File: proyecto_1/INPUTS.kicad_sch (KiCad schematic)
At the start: 28 parts, among them U10 FODM2705, U7 FODM2705, U8 FODM2705, U9 FODM2705

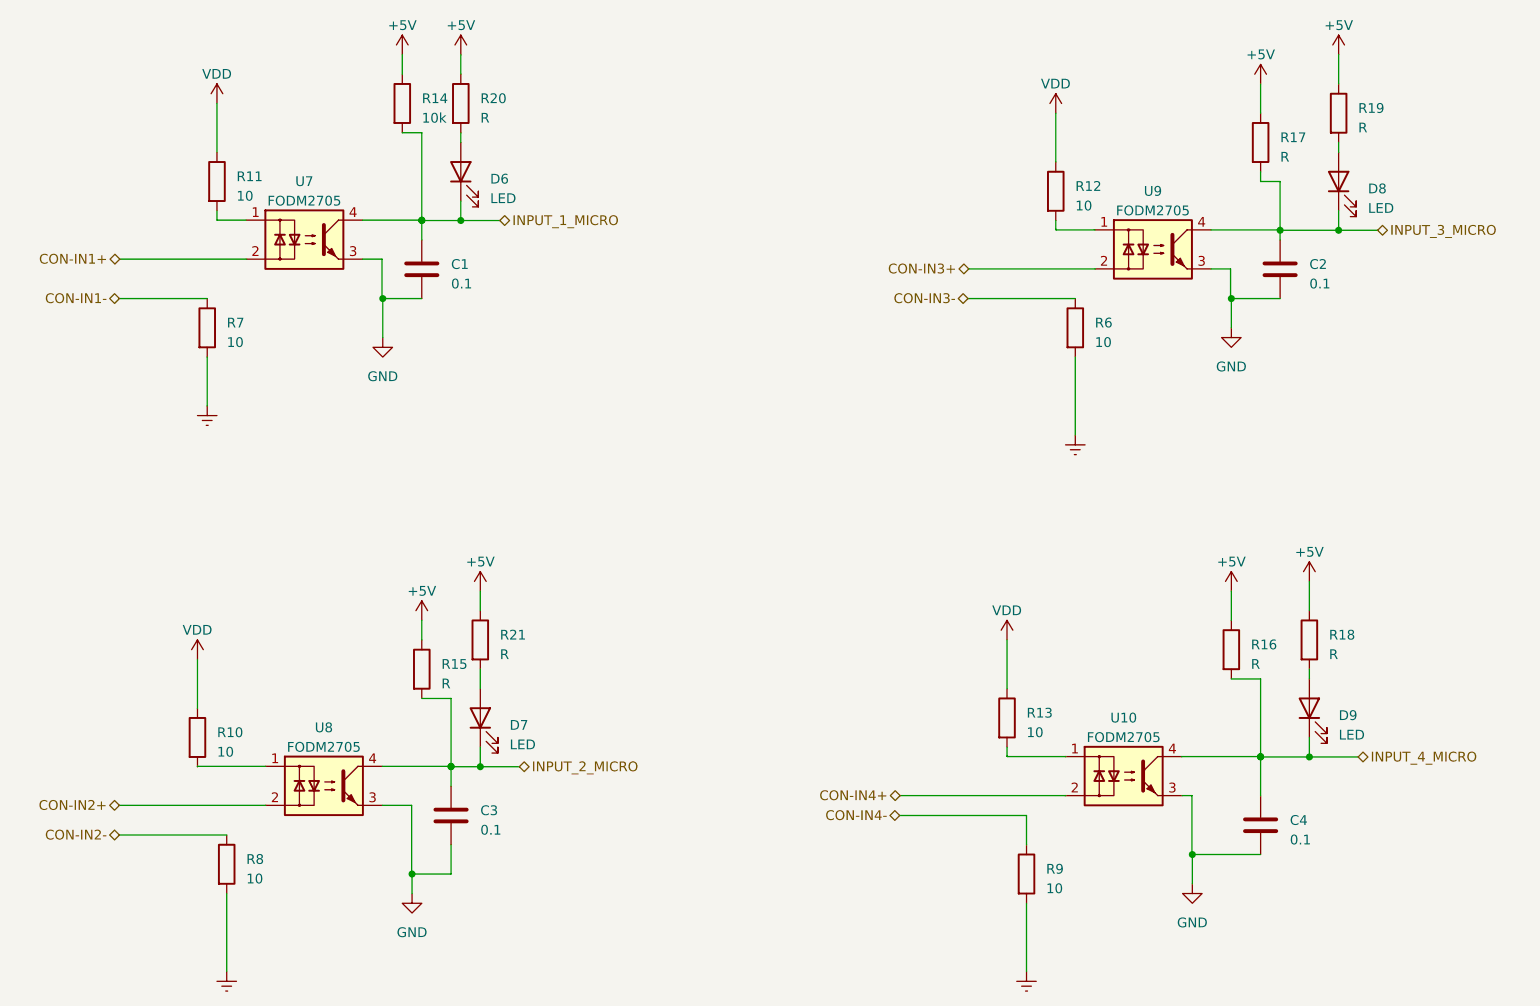
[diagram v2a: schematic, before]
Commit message: avance del proyecto
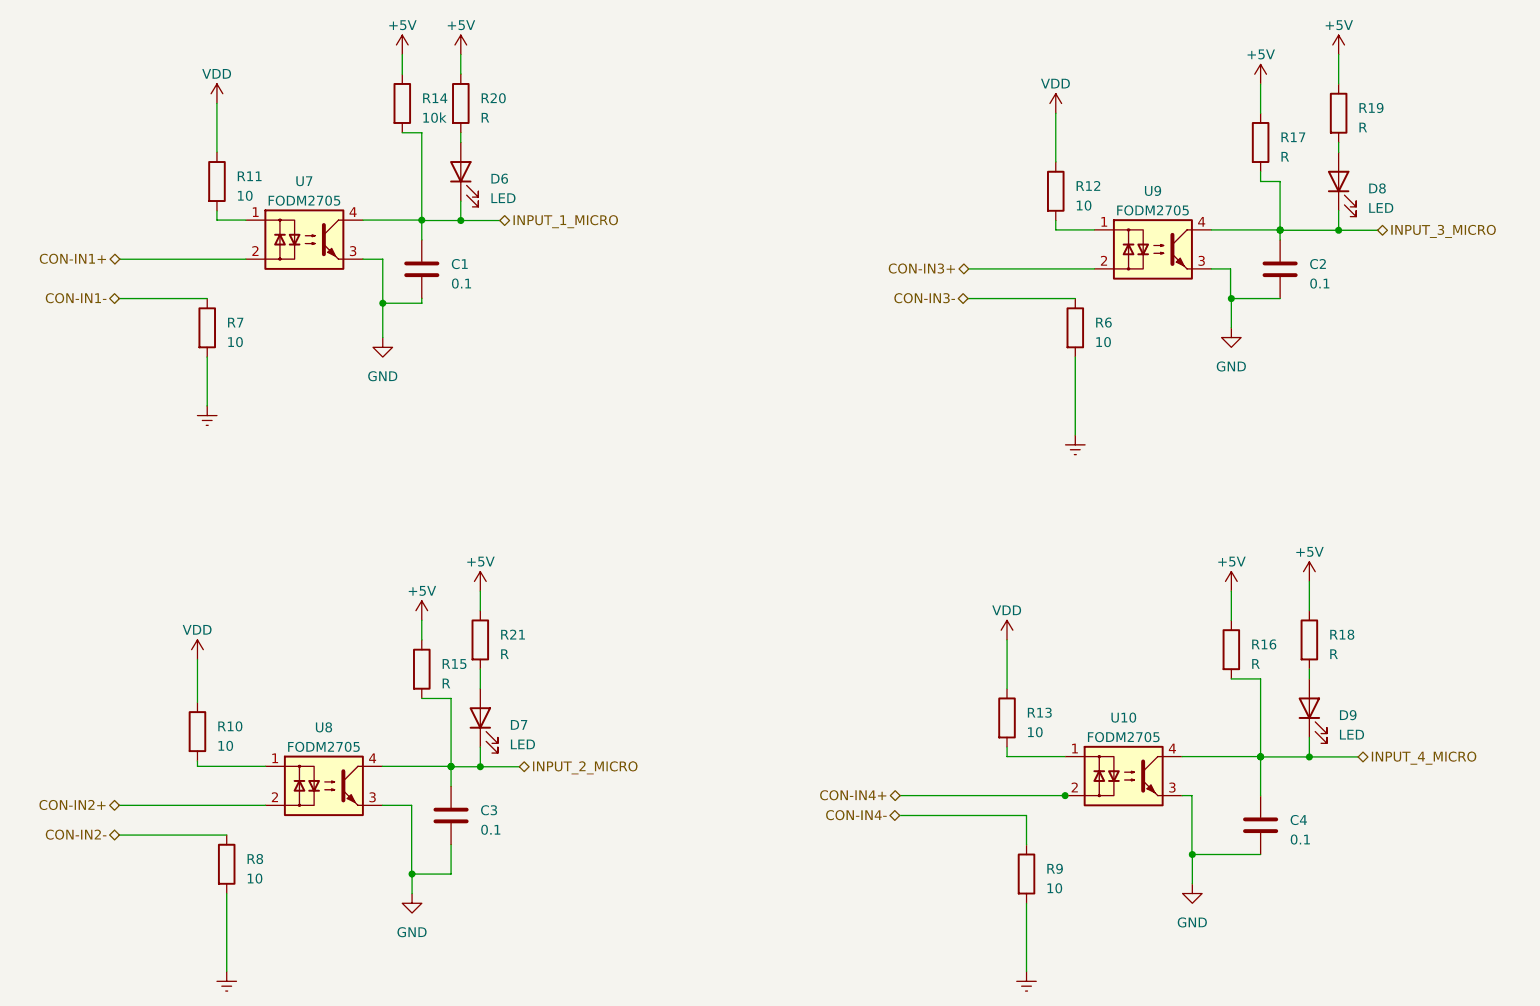
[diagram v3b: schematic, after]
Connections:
- net CON-IN1+: now also U7.2
- net CON-IN2+: now also U8.2
- net CON-IN3+: now also U9.2
- net CON-IN4+: now also U10.2
- net GND: now also U7.3, U9.3
- net INPUT_1_MICRO: no longer C1.1, R14.2
- net INPUT_3_MICRO: now also U9.4
- net INPUT_4_MICRO: now also U10.4
- net at U7.1: now also R11.2
- net at U7.4: now also C1.1, R14.2
- net at R12.2: now also U9.1
- net at R13.2: now also U10.1
- net at U8.1: now also R10.2
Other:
- moved on the sheet: R10
